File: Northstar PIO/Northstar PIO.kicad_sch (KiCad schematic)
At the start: 39 parts, among them J1 Conn_01x02, J1A1 Configuration Header, J2 Conn_01x02, J3 Conn_01x02, J4 Conn_01x02, J5 Conn_01x02, J6 Conn_01x02, J7 Conn_02x15_Odd_Even, P1 INPUT PORT, P2 OUTPUT PORT, U1B1 74LS74, U1C1 74LS74, U1D1 SN74LS164N, U2A1 74LS32, U2B1 74LS138, U2C1 74LS175, U2D1 74LS03, U2E1 74LS367, U3A1 74LS14, U3B1 74LS37, U3C1 74LS373, U3D1 74LS373

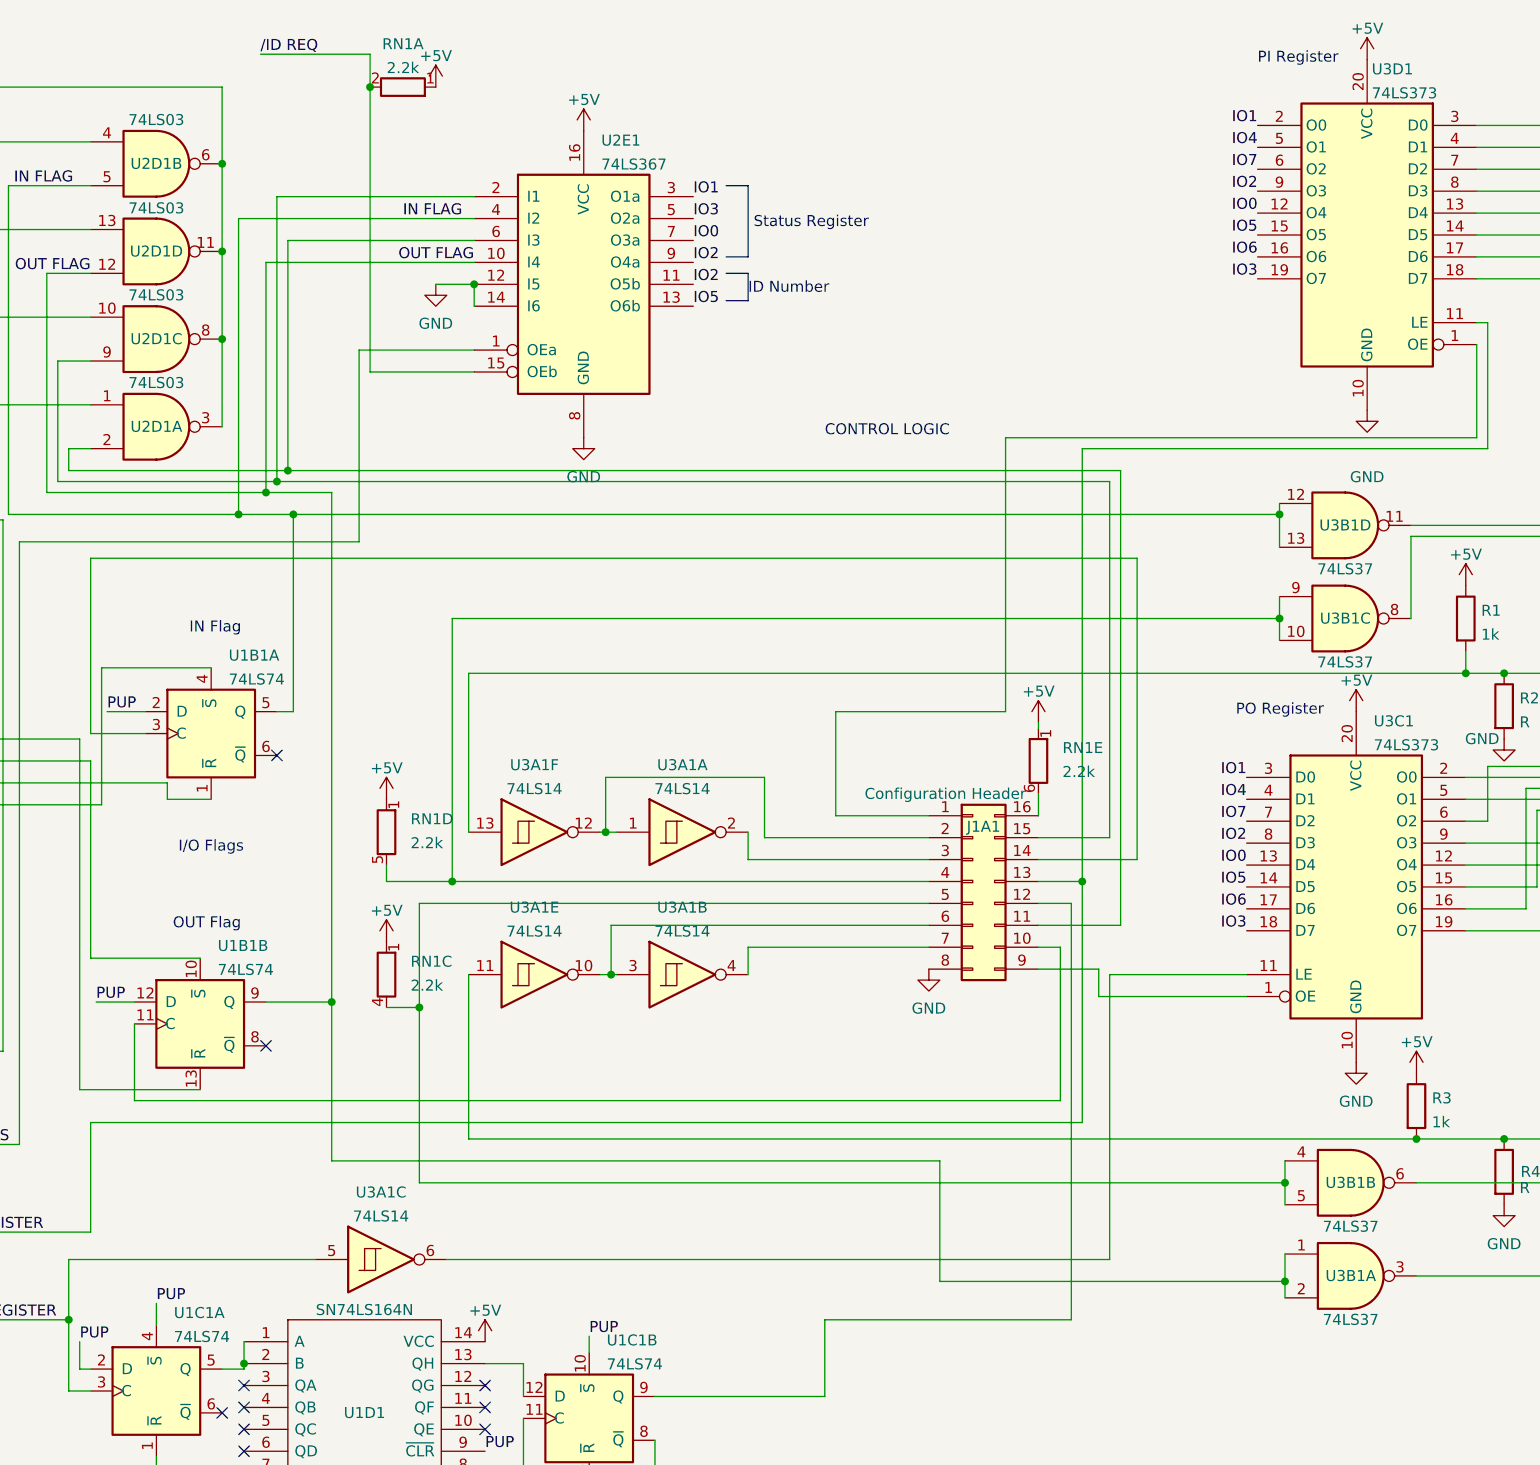
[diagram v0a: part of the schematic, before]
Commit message: small updates to boards
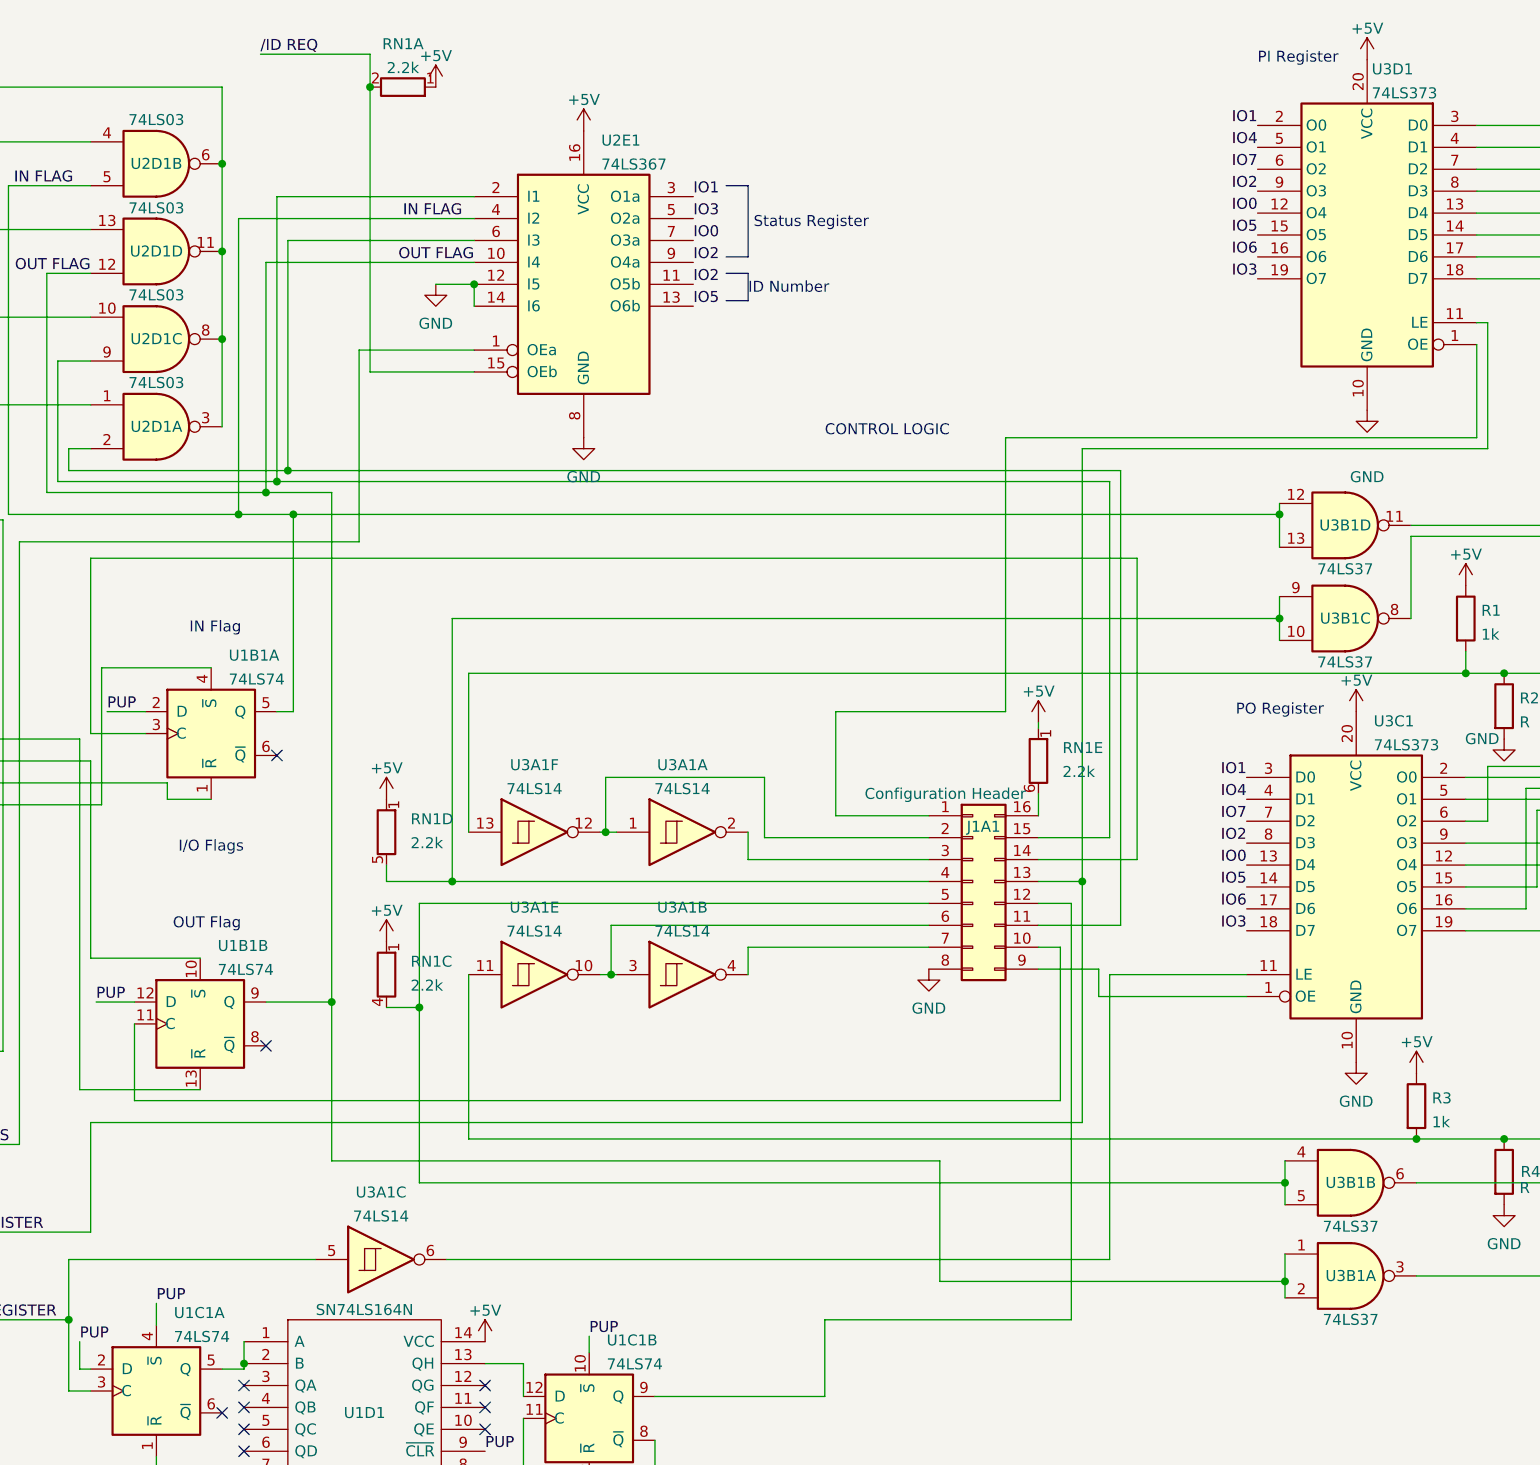
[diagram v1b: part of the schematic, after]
